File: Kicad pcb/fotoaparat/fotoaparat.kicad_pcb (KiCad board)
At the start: 2 copper layers, 128 x 93 mm, 73 parts, among them IC1 Lineární Regulátor, IC3 Lineární Regulátor Displaye, J3 LCD konektor, J4 Baterie, J7 Kamera, J9 Conn_01x11_Socket, U1 STM32L496RETx, U2 MCP73833-FCI/UN, Y1 8mhz krystal

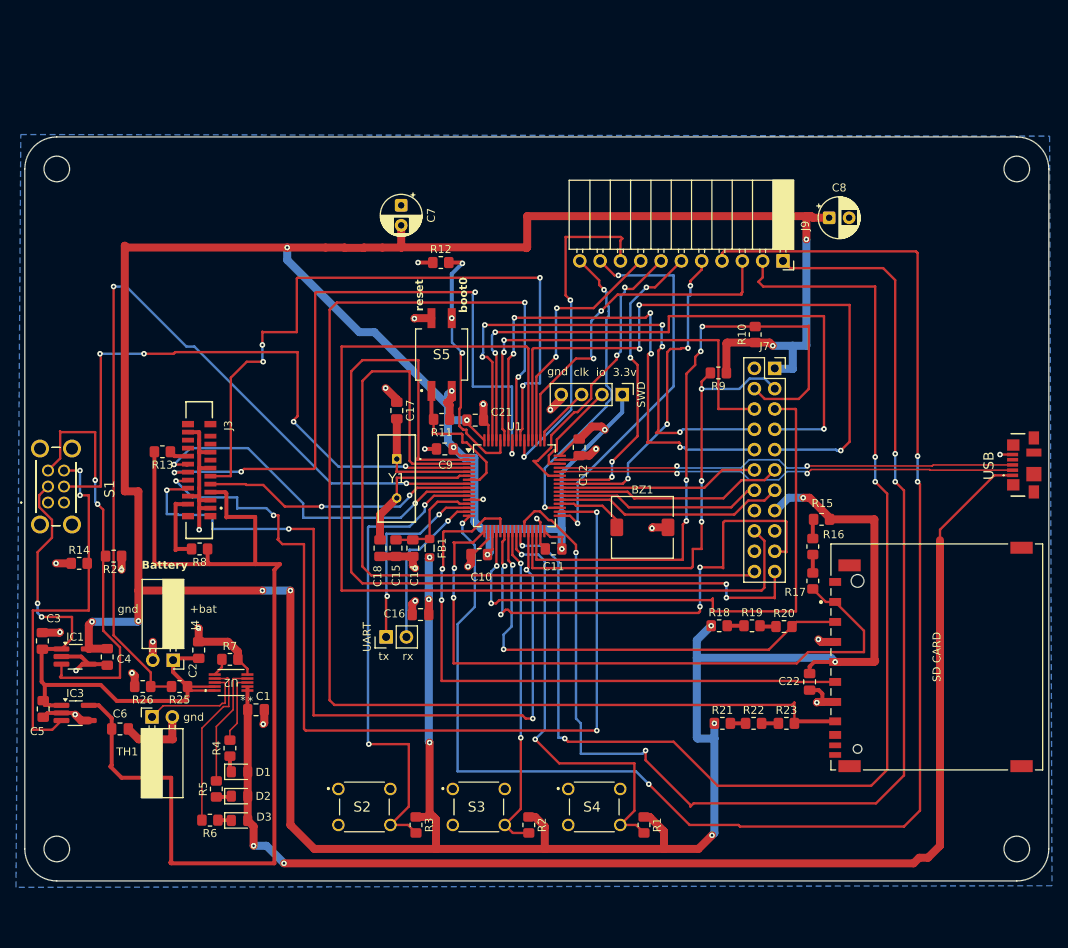
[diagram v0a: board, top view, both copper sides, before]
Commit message: Úprava designu
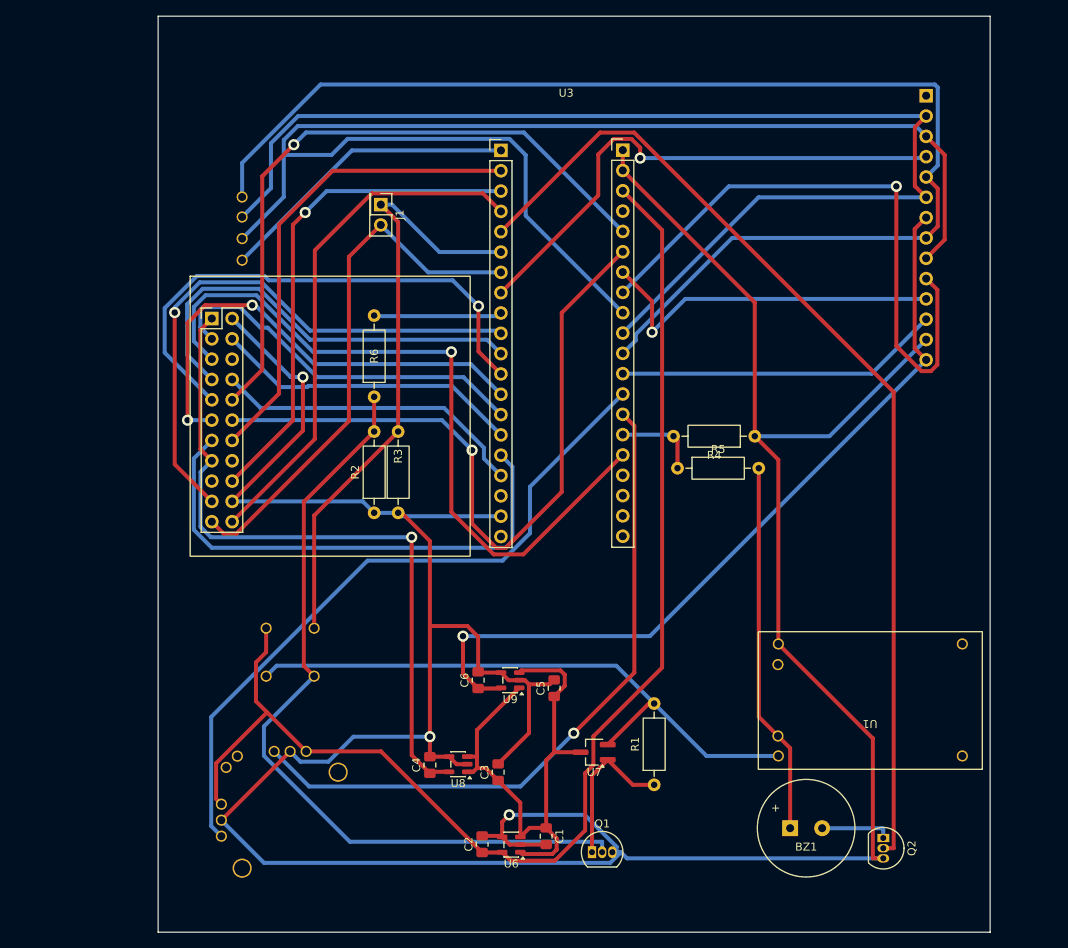
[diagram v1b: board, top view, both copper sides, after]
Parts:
- removed C10, C11, C12, C14, C21, C9: 100n, Capacitor_SMD:C_0805_2012Metric_Pad1.18x1.45mm_HandSolder
- removed C15, C16, C22: 1u, Capacitor_SMD:C_0805_2012Metric_Pad1.18x1.45mm_HandSolder
- removed C17, C18: 30p, Capacitor_SMD:C_0805_2012Metric_Pad1.18x1.45mm_HandSolder
- removed C7, C8: 10u, Capacitor_THT:CP_Radial_D5.0mm_P2.50mm
- removed D1, D2, D3: LED, LED_SMD:LED_0805_2012Metric_Pad1.15x1.40mm_HandSolder
- removed FB1: 120R, Inductor_SMD:L_0805_2012Metric_Pad1.05x1.20mm_HandSolder
- removed H1, H2, H3, H4: MountingHole, MountingHole:MountingHole_3.2mm_M3
- removed IC1: Lineární Regulátor, Package_TO_SOT_SMD:TSOT-23-5_HandSoldering
- removed IC3: Lineární Regulátor Displaye, Package_TO_SOT_SMD:TSOT-23-5_HandSoldering
- removed J3: LCD konektor, FFC2A32-20-T:GCT_FFC2A32-20-T
- removed J4: Baterie, Connector_PinSocket_2.54mm:PinSocket_1x02_P2.54mm_Horizontal
- removed J7: Kamera, Connector_PinSocket_2.54mm:PinSocket_2x11_P2.54mm_Vertical
- removed J9: Conn_01x11_Socket, Connector_PinSocket_2.54mm:PinSocket_1x11_P2.54mm_Horizontal
- removed R10, R11, R12, R13, R14, R15, R16, R17, R18, R19, R20, R21, R22, R23, R24, R26, R9: 4.7k, Resistor_SMD:R_0805_2012Metric_Pad1.20x1.40mm_HandSolder
- removed R25, R7: 1k, Resistor_SMD:R_0805_2012Metric_Pad1.20x1.40mm_HandSolder
- removed R8: 2, Resistor_SMD:R_0805_2012Metric_Pad1.20x1.40mm_HandSolder
- removed S1: Zapínací spínač, mfs:MFS201N24Z
- removed S2: tlačítko doleva, mc3:MC32829
- removed S3: prostřední tlačítko, mc3:MC32829
- removed S4: tlačítko doprava, mc3:MC32829
- removed S5: spínač, cfs201mb:CFS0201MB
- removed SD CARD: GSD090012SEU, gsd09:GSD090012SEU_AMP
- removed SWD: SWD, Connector_PinHeader_2.54mm:PinHeader_1x04_P2.54mm_Vertical
- removed TH1: 10k, Connector_PinSocket_2.54mm:PinSocket_1x02_P2.54mm_Horizontal
- removed UART: UART, Connector_PinHeader_2.54mm:PinHeader_1x02_P2.54mm_Vertical
- removed USB: USB Konektor, 47436:473460001
- removed Y1: 8mhz krystal, hc4:HC49S830507030ATF
- added J1: Conn_02x01, Connector_PinHeader_2.54mm:PinHeader_2x01_P2.54mm_Vertical, F.Cu at (125.5, 64.5)
- added Q1: BC547, Package_TO_SOT_THT:TO-92_Inline, F.Cu at (151.9, 145.4)
- added Q2: BC547, Package_TO_SOT_THT:TO-92_Inline, F.Cu at (188.3, 143.6)
- added SW1: SW_Push_Dual, Tlačítko:tlačítko 6x6x12, B.Cu at (117.3, 123.4)
- added U3: Stm32 Bluepill, Stm32 Bluepill:Bluepill, F.Cu at (140.0, 81.8)
- added U4: Lcd Display, Lcd Display:ili9341, B.Cu at (195.6, 96.8)
- added U5: FJ08k, Tlačítko:FJ08K-S, B.Cu at (120.2, 147.4)
- added U6: Me6211c, Package_TO_SOT_SMD:SOT-23-5, F.Cu at (141.8, 144.5)
- added U7: VBsemi SI2312CDS-T1-GE3, Package_TO_SOT_SMD:SOT-23W_Handsoldering, F.Cu at (152.2, 132.9)
- added U8: Me6211c, Package_TO_SOT_SMD:SOT-23-5, F.Cu at (135.2, 134.4)
- added U9: Me6211c, Package_TO_SOT_SMD:SOT-23-5, F.Cu at (141.7, 123.9)
- BZ1: footprint Inductor_SMD:L_SXN_SMDRI73 -> Jiangsu:Jiangsu
- C1, C2, C3, C4, C5, C6: value 1u -> 4.7uf
- R1, R2: value 4.7k -> 100k; footprint Resistor_SMD:R_0805_2012Metric_Pad1.20x1.40mm_HandSolder -> Resistor_THT:R_Axial_DIN0207_L6.3mm_D2.5mm_P10.16mm_Horizontal
- R3: value 4.7k -> 10k; footprint Resistor_SMD:R_0805_2012Metric_Pad1.20x1.40mm_HandSolder -> Resistor_THT:R_Axial_DIN0207_L6.3mm_D2.5mm_P10.16mm_Horizontal
- R4: value 1k -> 100k; footprint Resistor_SMD:R_0805_2012Metric_Pad1.20x1.40mm_HandSolder -> Resistor_THT:R_Axial_DIN0207_L6.3mm_D2.5mm_P10.16mm_Horizontal
- R5: value 1k -> 30k; footprint Resistor_SMD:R_0805_2012Metric_Pad1.20x1.40mm_HandSolder -> Resistor_THT:R_Axial_DIN0207_L6.3mm_D2.5mm_P10.16mm_Horizontal
- R6: value 1k -> 50k; footprint Resistor_SMD:R_0805_2012Metric_Pad1.20x1.40mm_HandSolder -> Resistor_THT:R_Axial_DIN0207_L6.3mm_D2.5mm_P10.16mm_Horizontal
- U1: value STM32L496RETx -> TP4056; footprint Package_QFP:LQFP-64_10x10mm_P0.5mm -> TP4056:TP4056
- U2: value MCP73833-FCI/UN -> ov7670 fifo; footprint MCP:MSOP10_MC_MCH -> ov7670:ov7670
- moved R4 76.3 mm to (172.2, 93.4), turned to 180 degrees
- moved R5 70.2 mm to (162.6, 97.4), turned to 0 degrees
- moved C5 63.9 mm to (147.2, 124.9), turned to 90 degrees
- moved U1 61.3 mm to (200.7, 117.8), turned to 180 degrees
- moved C3 59.3 mm to (140.2, 135.4)
- moved R6 56.8 mm to (124.7, 88.5), turned to 90 degrees
- moved BZ1 50.6 mm to (178.7, 151.1)
- moved C6 45.2 mm to (137.7, 123.9), turned to 90 degrees
- moved R2 43.5 mm to (124.7, 103.0), turned to 90 degrees
- moved C2 42.9 mm to (138.2, 144.4)
- moved C4 42.5 mm to (131.6, 134.5)
- moved C1 39.6 mm to (146.2, 143.4), turned to -90 degrees
- moved R3 39.1 mm to (127.7, 103.0), turned to 90 degrees
- moved U2 18.8 mm to (102.7, 105.8), turned to 0 degrees
- moved R1 5.17 mm to (159.7, 137.0), turned to 90 degrees
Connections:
- BZ1 pad 1: /buzzer -> +BATT
- BZ1 pad 2: GND -> Net-(BZ1--)
- C1 pad 1: VBUS -> +4V
- C2 pad 1: +BATT -> +3.3V
- C3 pad 1: +BATT -> +4V
- C4 pad 1: GND -> +3.3V ov7670
- C4 pad 2: +3.3V -> GND
- C5 pad 1: +BATT -> +4V
- C6 pad 1: GND -> +3.3V lcd
- C6 pad 2: +3.3V LCD -> GND
- R1 pad 1: +3.3V -> Net-(Q1-C)
- R1 pad 2: /sw3 -> Net-(U1-OUT+)
- R2 pad 1: +3.3V -> GND
- R2 pad 2: /sw2 -> Net-(Q1-B)
- R3 pad 1: +3.3V -> GND
- R3 pad 2: /sw1 -> /tx
- R4 pad 1: Net-(D1-K) -> GND
- R4 pad 2: Net-(U2-STAT1) -> Net-(U3-pa1)
- R5 pad 1: Net-(D2-K) -> Net-(U3-pa1)
- R5 pad 2: Net-(U2-STAT2) -> +BATT
- R6 pad 1: /Indikátor Nabíjení -> Net-(Q1-B)
- R6 pad 2: Net-(U2-*PG) -> Net-(U3-pa12)
- U1 pad 1: +3.3V -> unconnected-(U1-IN+-Pad1)
- U1 pad 2: /wrst -> unconnected-(U1-IN--Pad2)
- U1 pad 3: /rrst -> Net-(U1-OUT+)
- U1 pad 4: /Backlight Regulátor en -> GND
- U1 pad 5: /osc in -> +BATT
- U1 pad 6: /osc out -> -BATT
- U2 pad 1: VBUS -> +3.3V ov7670
- U2 pad 10: +BATT -> Net-(U2-d4)
- U2 pad 2: VBUS -> GND
- U2 pad 3: Net-(U2-STAT1) -> Net-(U2-sioc)
- U2 pad 4: Net-(U2-STAT2) -> Net-(U2-siod)
- U2 pad 5: GND -> Net-(U2-vsync)
- U2 pad 6: Net-(U2-PROG) -> unconnected-(U2-href-Pad6)
- U2 pad 7: Net-(U2-*PG) -> Net-(U2-d7)
- U2 pad 9: +BATT -> Net-(U2-d5)
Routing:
- net +3.3V: track 548.7 -> 161.0 mm, vias 21 -> 0
- net GND: track 118.3 -> 410.7 mm, vias 27 -> 3
- net /pa2: track 190.7 -> 0.00 mm, vias 4 -> 0
- net Net-(U3-pa7): track 0.00 -> 169.8 mm
- net Net-(U3-pa5): track 0.00 -> 160.4 mm
- net /pb1: track 159.6 -> 0.00 mm, vias 4 -> 0
- net VBUS: track 159.1 -> 0.00 mm, vias 2 -> 0
- net /sd miso: track 157.5 -> 0.00 mm, vias 2 -> 0
- net /pb0: track 152.4 -> 0.00 mm, vias 4 -> 0
- net Net-(U3-pa6): track 0.00 -> 150.3 mm
- net Net-(Q2-B): track 0.00 -> 126.0 mm
- net /rck: track 126.0 -> 0.00 mm
- net +3.3V LCD: track 125.4 -> 0.00 mm
- net /scl: track 115.3 -> 0.00 mm, vias 4 -> 0
- net /wrst: track 111.7 -> 0.00 mm, vias 2 -> 0
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- removed copper zone on B.Cu, net GND
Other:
- board size 128 x 93 mm -> 104 x 114.5 mm
- board text removed: "+bat"
- board text removed: "3.3v"
- board text removed: "Battery"
- board text removed: "Dat0 - 7"
- board text removed: "boot0"
- board text removed: "clk"
- board text removed: "gnd"
- board text removed: "href"
- board text removed: "io"
- board text removed: "nc"
- board text removed: "rck"
- board text removed: "reset"
- board text removed: "rrst"
- board text removed: "rx"
- board text removed: "scl"
- board text removed: "sda"
- board text removed: "tx"
- board text removed: "vsync"
- board text removed: "wr"
- board text removed: "wrst"
